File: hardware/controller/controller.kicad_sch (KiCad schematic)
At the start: 29 parts, among them J1 DC_12V_IN, J2 HDD_POWER_OUT, J3 470531000, J4 470531000, J6 FH19C-7S-0.5SH10, Q1 2N3904, Q2 2N3904, U1 TSR0.5-2450, U2 XIAO-RP2350-SMD, U3 INA228, U4 74HC4051

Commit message: update symbol and footprint libraries for thermistor strip
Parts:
- J6: footprint CONN7_FH19C_7S_HIR -> Hirose_FH19C_7S_0_5SH:CONN7_FH19C_7S_HIR
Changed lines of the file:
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@@
 			)
 		)
-		(property "Footprint" "CONN7_FH19C_7S_HIR"
+		(property "Footprint" "Hirose_FH19C_7S_0_5SH:CONN7_FH19C_7S_HIR"
 			(at 213.36 124.46 0)
 			(hide yes)

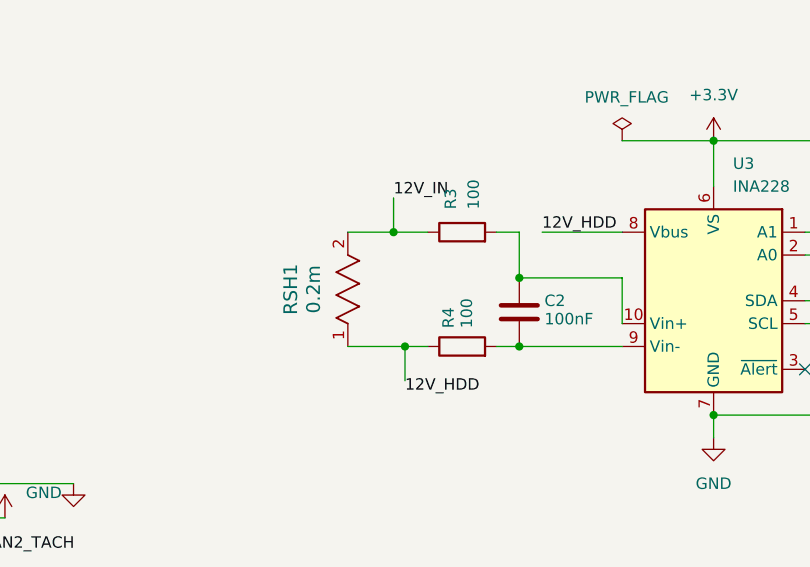
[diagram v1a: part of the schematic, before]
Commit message: fix shunt footprint
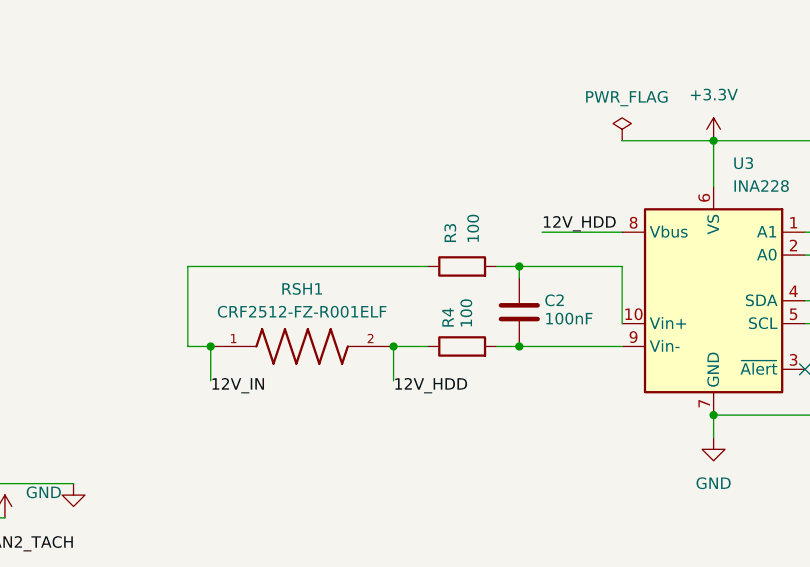
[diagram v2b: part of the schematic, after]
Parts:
- removed RSH1: 0.2m, CSS2H_3920R_L200F:RES_3920R_L200x_BRN, symbol CSS2H_3920R_L200F:CSS2H-3920R-L200F
- added RSH1: CRF2512-FZ-R001ELF, CRF2512-FZ-R001ELF:RESC6432X80N, symbol CRF2512-FZ-R001ELF:CRF2512-FZ-R001ELF
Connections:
- net 12V_HDD: now also RSH1.2
- net 12V_IN: now also RSH1.1
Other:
- moved on the sheet: R3
